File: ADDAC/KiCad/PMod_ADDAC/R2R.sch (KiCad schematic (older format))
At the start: 24 parts, among them J1 Conn_01x12_Male, U2 TL072

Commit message: Schematic
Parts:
- J1: footprint Connector_PinHeader_2.54mm:PinHeader_2x06_P2.54mm_Horizontal -> Connector_PinHeader_2.54mm:PinHeader_2x06_P2.54mm_Vertical
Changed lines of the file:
@@
 F 0 "J1" H 1208 3889 50  0000 C CNN
 F 1 "Conn_01x12_Male" H 1208 3890 50  0001 C CNN
-F 2 "Connector_PinHeader_2.54mm:PinHeader_2x06_P2.54mm_Horizontal" H 1100 3300 50  0001 C CNN
+F 2 "Connector_PinHeader_2.54mm:PinHeader_2x06_P2.54mm_Vertical" H 1100 3300 50  0001 C CNN
 F 3 "~" H 1100 3300 50  0001 C CNN
 	1    1100 3300

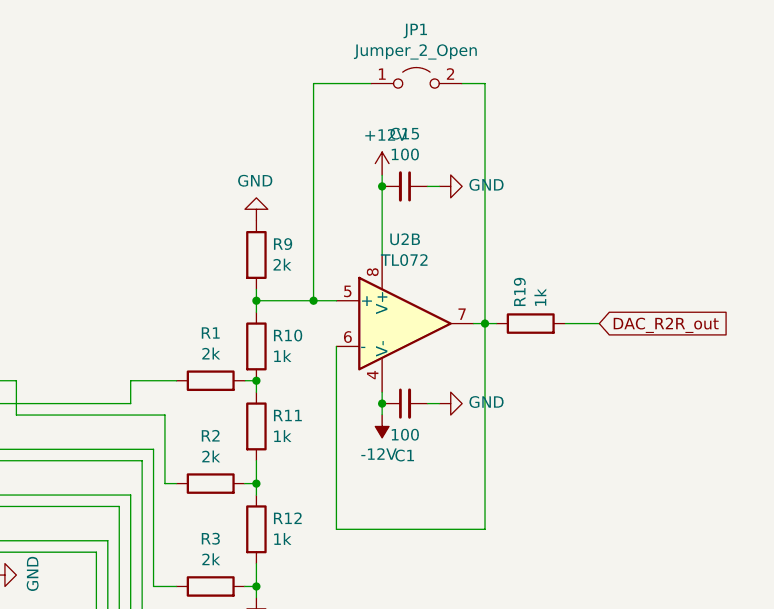
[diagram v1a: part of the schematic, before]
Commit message: Arduino tests
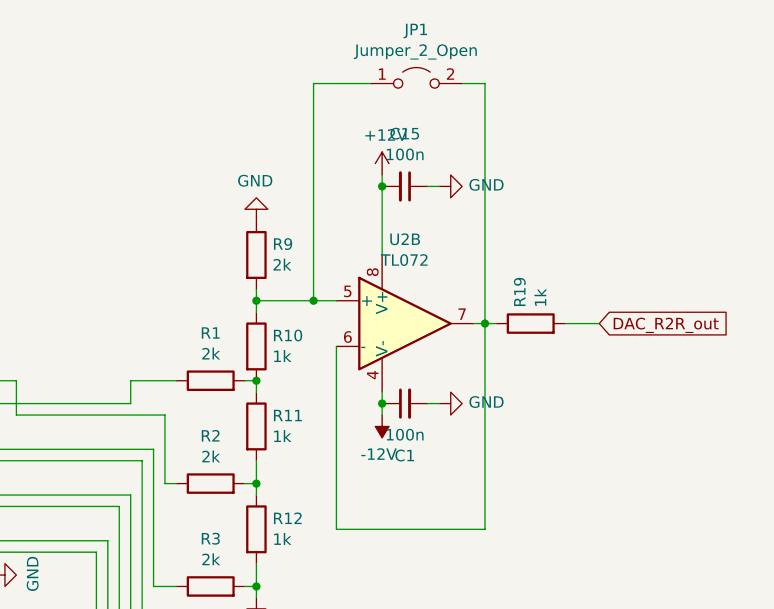
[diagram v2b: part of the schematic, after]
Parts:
- C1, C15: value 100 -> 100n
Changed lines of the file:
@@
 AR Path="/6242AFE6/6243F824" Ref="C1"  Part="1"
 F 0 "C1" V 2921 2800 50  0000 C CNN
-F 1 "100" V 3012 2800 50  0000 C CNN
+F 1 "100n" V 3012 2800 50  0000 C CNN
 F 2 "Capacitor_SMD:C_0805_2012Metric_Pad1.15x1.40mm_HandSolder" H 3150 2800 50  0001 C CNN
 F 3 "~" H 3150 2800 50  0001 C CNN
@@
 	1    0    0    -1
 $EndComp
-Wire Wire Line
-	3300 1850 3250 1850
 $Comp
 L power:GND #PWR?
@@
 	0    -1   -1   0
 $EndComp
-Wire Wire Line
-	3050 1850 3050 1800
-Connection ~ 3050 1850
-$Comp
-L Device:C_Small C?
-U 1 1 624B430E
-P 3150 1850
-AR Path="/624B430E" Ref="C?"  Part="1"
-AR Path="/6242AFE6/624B430E" Ref="C15"  Part="1"
-F 0 "C15" V 2921 1850 50  0000 C CNN
-F 1 "100" V 3012 1850 50  0000 C CNN
-F 2 "Capacitor_SMD:C_0805_2012Metric_Pad1.15x1.40mm_HandSolder" H 3150 1850 50  0001 C CNN
-F 3 "~" H 3150 1850 50  0001 C CNN
-	1    3150 1850
-	0    1    1    0
-$EndComp
 $Comp
 L Amplifier_Operational:TL072 U?
@@
 	1    0    0    -1
 $EndComp
-Wire Wire Line
-	3050 1850 3050 2150
 $Comp
 L power:+12V #PWR015
@@
 	0    1    1    0
 $EndComp
+Connection ~ 3050 1850
+Wire Wire Line
+	3050 1850 3050 2150
+Wire Wire Line
+	3050 1850 3050 1800
+$Comp
+L Device:C_Small C?
+U 1 1 624B430E
+P 3150 1850
+AR Path="/624B430E" Ref="C?"  Part="1"
+AR Path="/6242AFE6/624B430E" Ref="C15"  Part="1"
+F 0 "C15" V 2921 1850 50  0000 C CNN
+F 1 "100n" V 3012 1850 50  0000 C CNN
+F 2 "Capacitor_SMD:C_0805_2012Metric_Pad1.15x1.40mm_HandSolder" H 3150 1850 50  0001 C CNN
+F 3 "~" H 3150 1850 50  0001 C CNN
+	1    3150 1850
+	0    1    1    0
+$EndComp
+Wire Wire Line
+	3300 1850 3250 1850
 $EndSCHEMATC
